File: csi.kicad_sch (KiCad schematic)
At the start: 0 parts

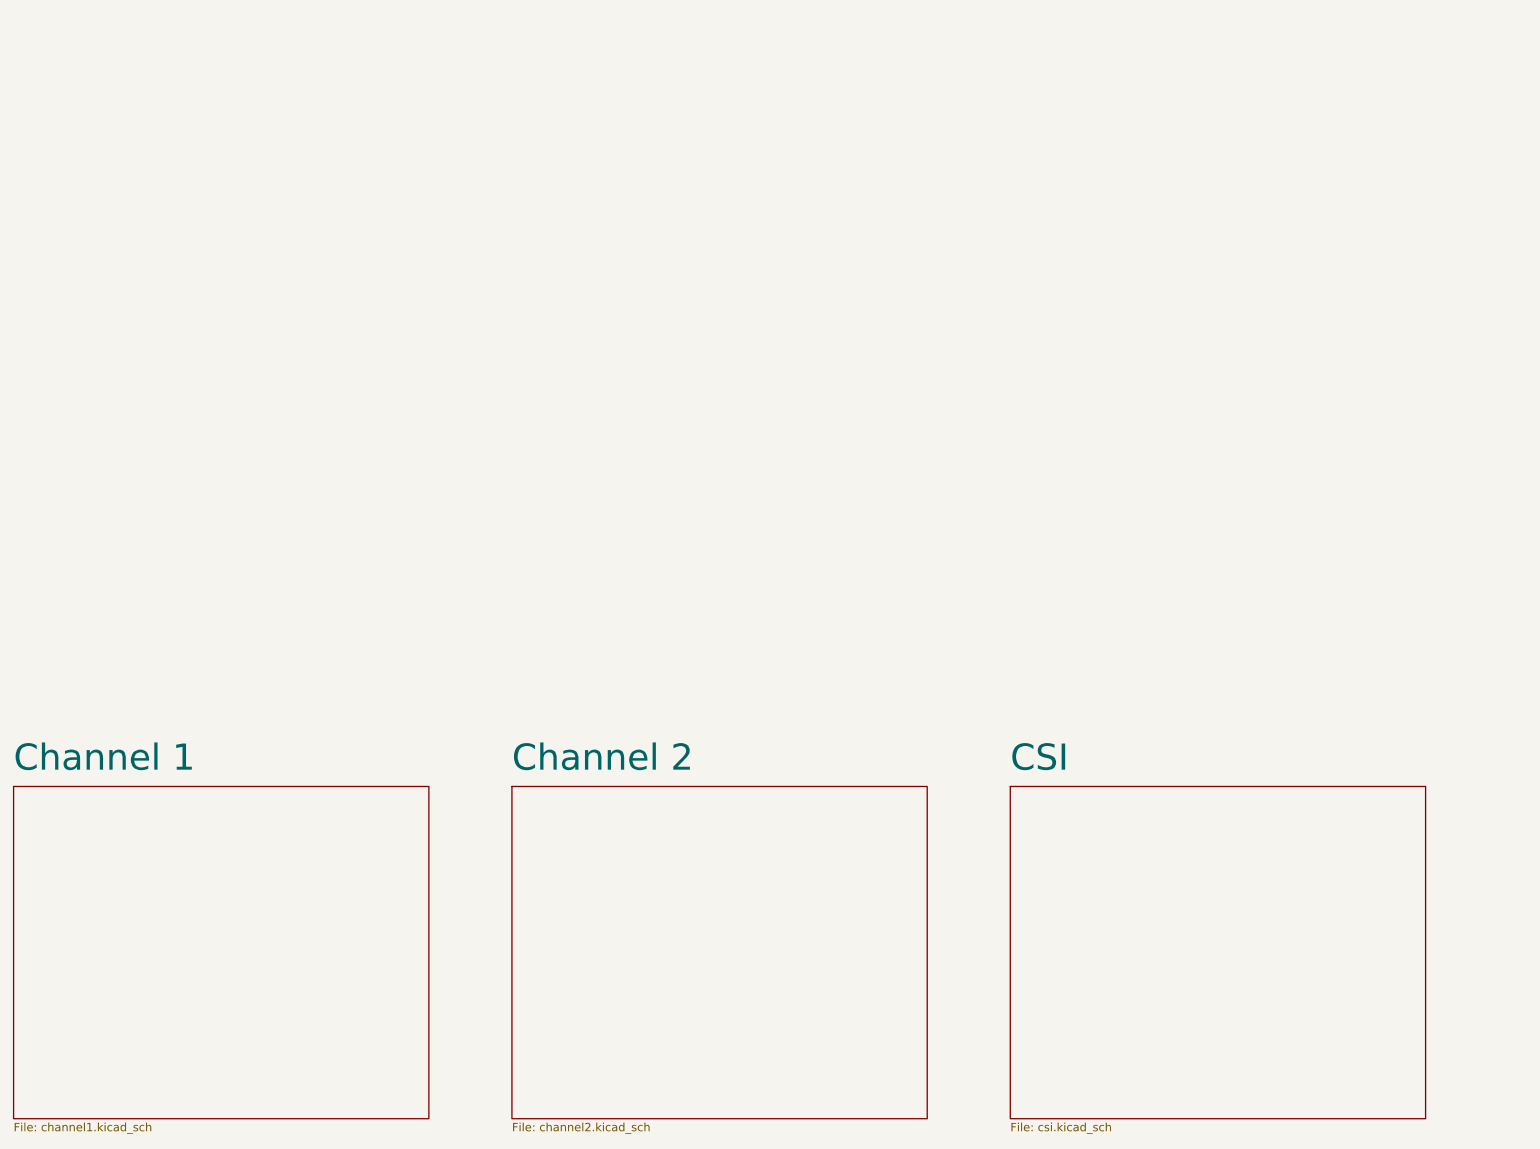
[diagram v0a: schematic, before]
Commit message: Schematic cleanup
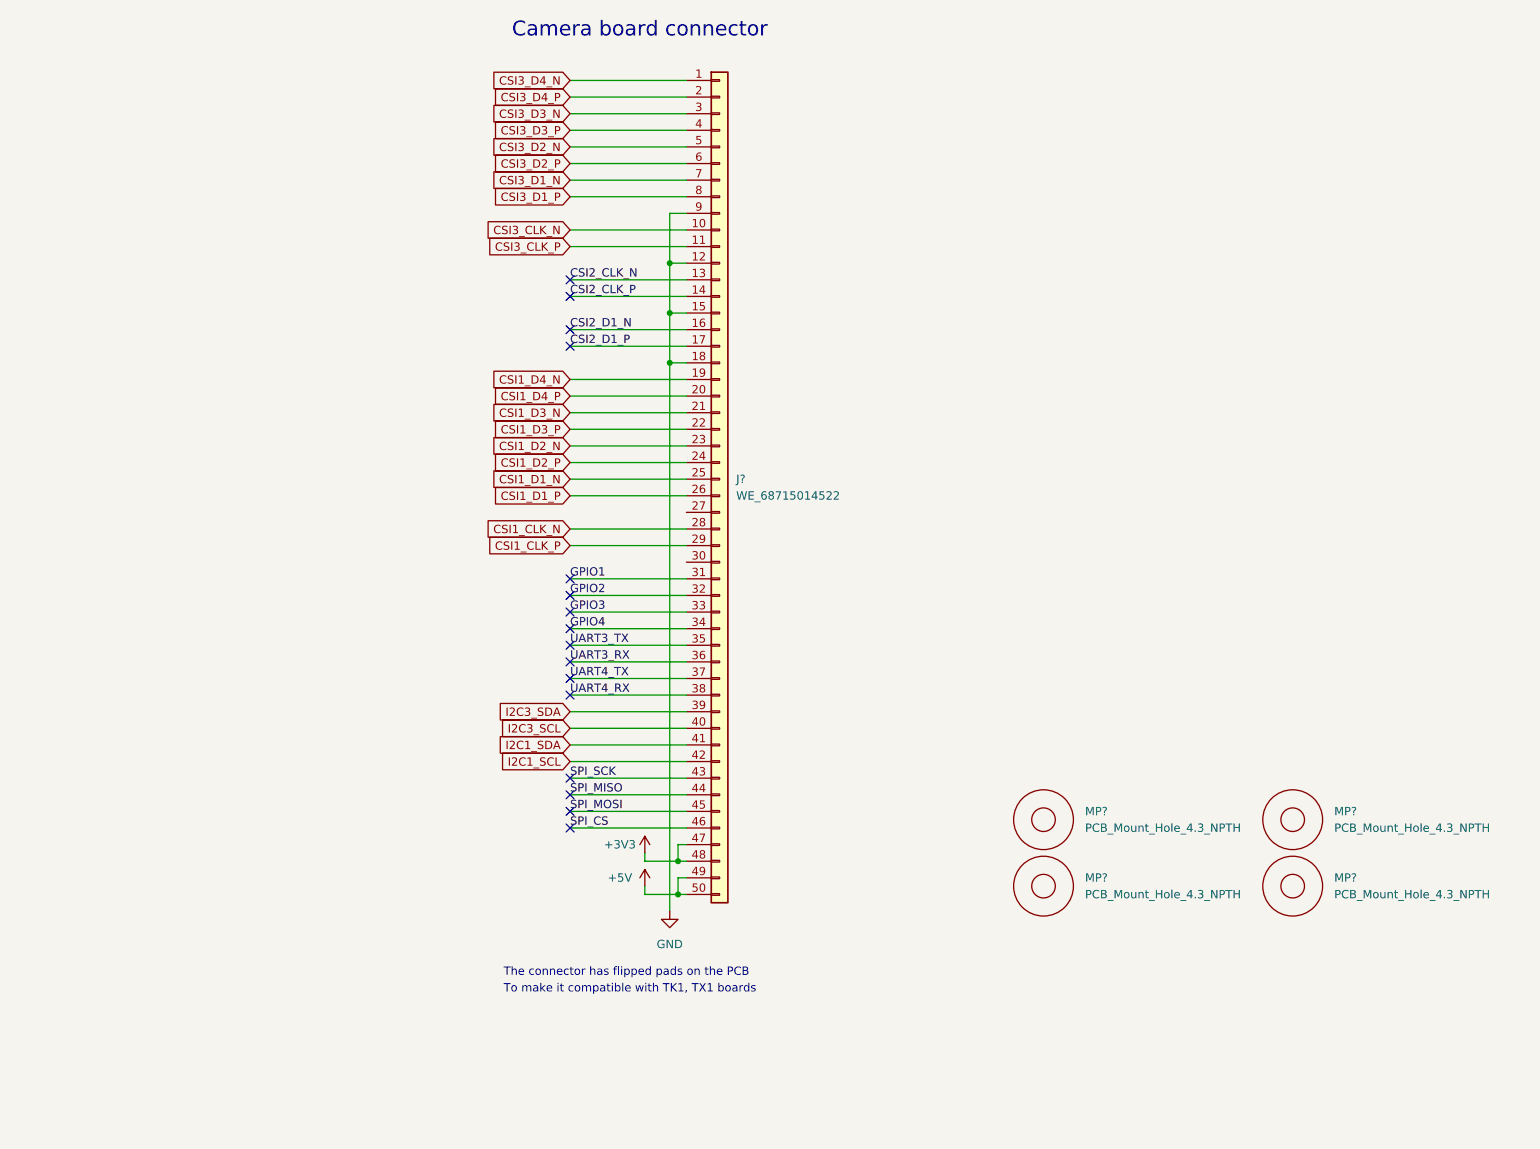
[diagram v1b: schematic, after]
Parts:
- added J?: WE_68715014522, antmicro-footprints:WE_68715014522, symbol antmicroFCCConnectors:WE_68715014522
- added MP? (x4): PCB_Mount_Hole_4.3_NPTH, antmicro-footprints:mounting-hole-4.2mm-NPTH, symbol antmicroMechanicalParts:PCB_Mount_Hole_4.3_NPTH
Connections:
- new net +3V3: J?.47 (Pin_47), J?.48 (Pin_48)
- new net +5V: J?.49 (Pin_49), J?.50 (Pin_50)
- new net CSI1_CLK_N: J?.28 (Pin_28)
- new net CSI1_CLK_P: J?.29 (Pin_29)
- new net CSI1_D1_N: J?.25 (Pin_25)
- new net CSI1_D1_P: J?.26 (Pin_26)
- new net CSI1_D2_N: J?.23 (Pin_23)
- new net CSI1_D2_P: J?.24 (Pin_24)
- new net CSI1_D3_N: J?.21 (Pin_21)
- new net CSI1_D3_P: J?.22 (Pin_22)
- new net CSI1_D4_N: J?.19 (Pin_19)
- new net CSI1_D4_P: J?.20 (Pin_20)
- new net CSI2_CLK_N: J?.13 (Pin_13)
- new net CSI2_CLK_P: J?.14 (Pin_14)
- new net CSI2_D1_N: J?.16 (Pin_16)
- new net CSI2_D1_P: J?.17 (Pin_17)
- new net CSI3_CLK_N: J?.10 (Pin_10)
- new net CSI3_CLK_P: J?.11 (Pin_11)
- new net CSI3_D1_N: J?.7 (Pin_7)
- new net CSI3_D1_P: J?.8 (Pin_8)
- new net CSI3_D2_N: J?.5 (Pin_5)
- new net CSI3_D2_P: J?.6 (Pin_6)
- new net CSI3_D3_N: J?.3 (Pin_3)
- new net CSI3_D3_P: J?.4 (Pin_4)
- new net CSI3_D4_N: J?.1 (Pin_1)
- new net CSI3_D4_P: J?.2 (Pin_2)
- new net GND: J?.12 (Pin_12), J?.15 (Pin_15), J?.18 (Pin_18), J?.9 (Pin_9)
- new net GPIO1: J?.31 (Pin_31)
- new net GPIO2: J?.32 (Pin_32)
- new net GPIO3: J?.33 (Pin_33)
- new net GPIO4: J?.34 (Pin_34)
- new net I2C1_SCL: J?.42 (Pin_42)
- new net I2C1_SDA: J?.41 (Pin_41)
- new net I2C3_SCL: J?.40 (Pin_40)
- new net I2C3_SDA: J?.39 (Pin_39)
- new net SPI_CS: J?.46 (Pin_46)
- new net SPI_MISO: J?.44 (Pin_44)
- new net SPI_MOSI: J?.45 (Pin_45)
- new net SPI_SCK: J?.43 (Pin_43)
- new net UART3_RX: J?.36 (Pin_36)
- new net UART3_TX: J?.35 (Pin_35)
- new net UART4_RX: J?.38 (Pin_38)
- new net UART4_TX: J?.37 (Pin_37)
- no-connect marks 0 -> 16
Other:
- removed sheet CSI
- removed sheet Channel 1
- removed sheet Channel 2
- note added: "Camera board connector"
- note added: "The connector has flipped pads on the PCB"
- note added: "To make it compatible with TK1, TX1 boards"
- title: Antmicro HDMI MIPI Bridge -> (none)
